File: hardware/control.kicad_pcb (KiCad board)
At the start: 2 copper layers, 49 parts, among them P1 POWER, P2 POWER, P3 DATA, P4 DATA, P5 ISP, P6 CONN_1, P7 CONN_1, P8 DISPLAY, P9 I2C, Q1 NX2301P, Q10 NX2301P, Q11 NX2301P, Q12 NX2301P, Q13 NX2301P, Q14 NX2301P, Q15 NX2301P, Q16 NX2301P, Q2 NX2301P, Q3 NX2301P, Q4 NX2301P, Q5 NX2301P, Q6 NX2301P, Q7 NX2301P, Q8 NX2301P, Q9 NX2301P, SW1 RESET, U1 AP1509, U2 ATMEGA328P-P, U3 74HC138, U4 74HC138, U5 TLC5940, X1 16MHz

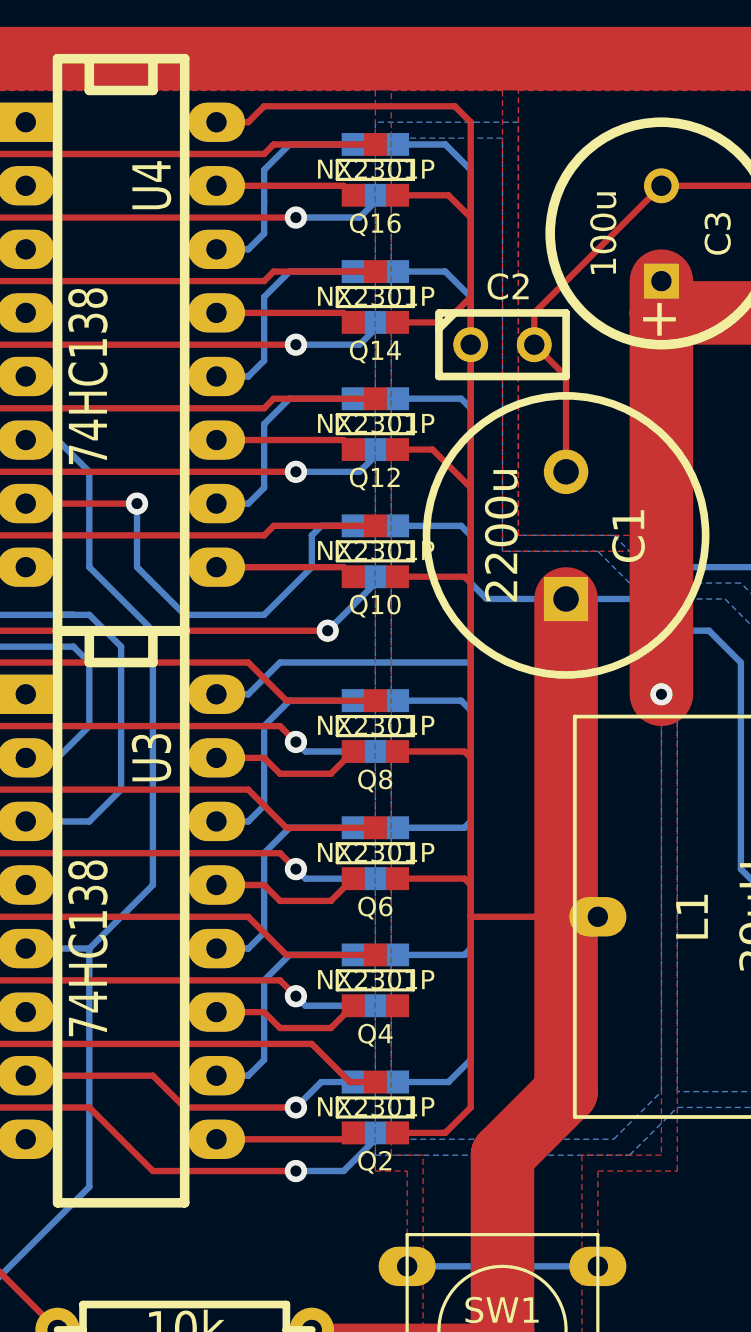
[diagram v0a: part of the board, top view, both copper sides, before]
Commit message: Final hardware tweaks.
Signed-off-by: Paul Brook <paul@nowt.org>
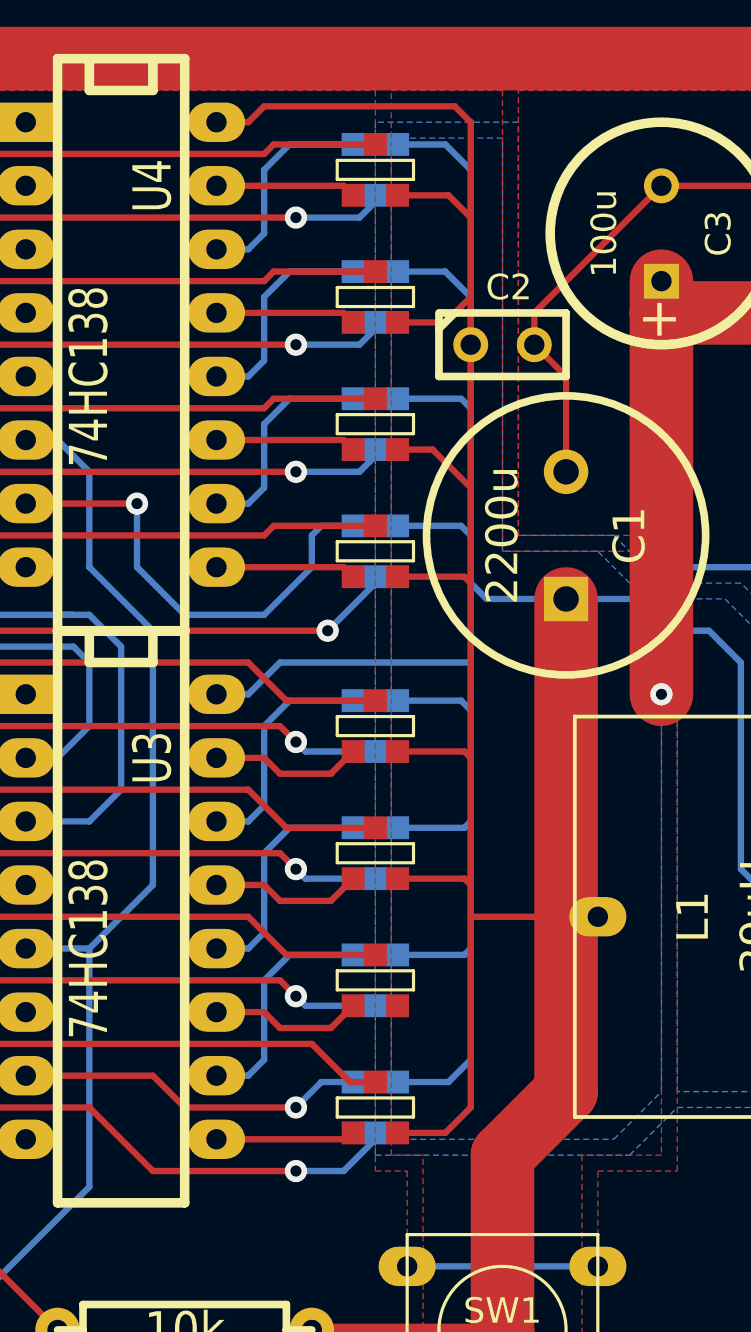
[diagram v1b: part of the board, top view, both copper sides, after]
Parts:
- Q1, Q10, Q11, Q12, Q13, Q14, Q15, Q16, Q2, Q3, Q4, Q5, Q6, Q7, Q8, Q9: footprint SOT23GDS -> SOT23GDS_NP
